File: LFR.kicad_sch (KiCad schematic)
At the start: 6 parts, among them M1 Motor_DC, M2 Motor_DC, U1 ESP32-S2-WROVER, U2 DRV8833PW

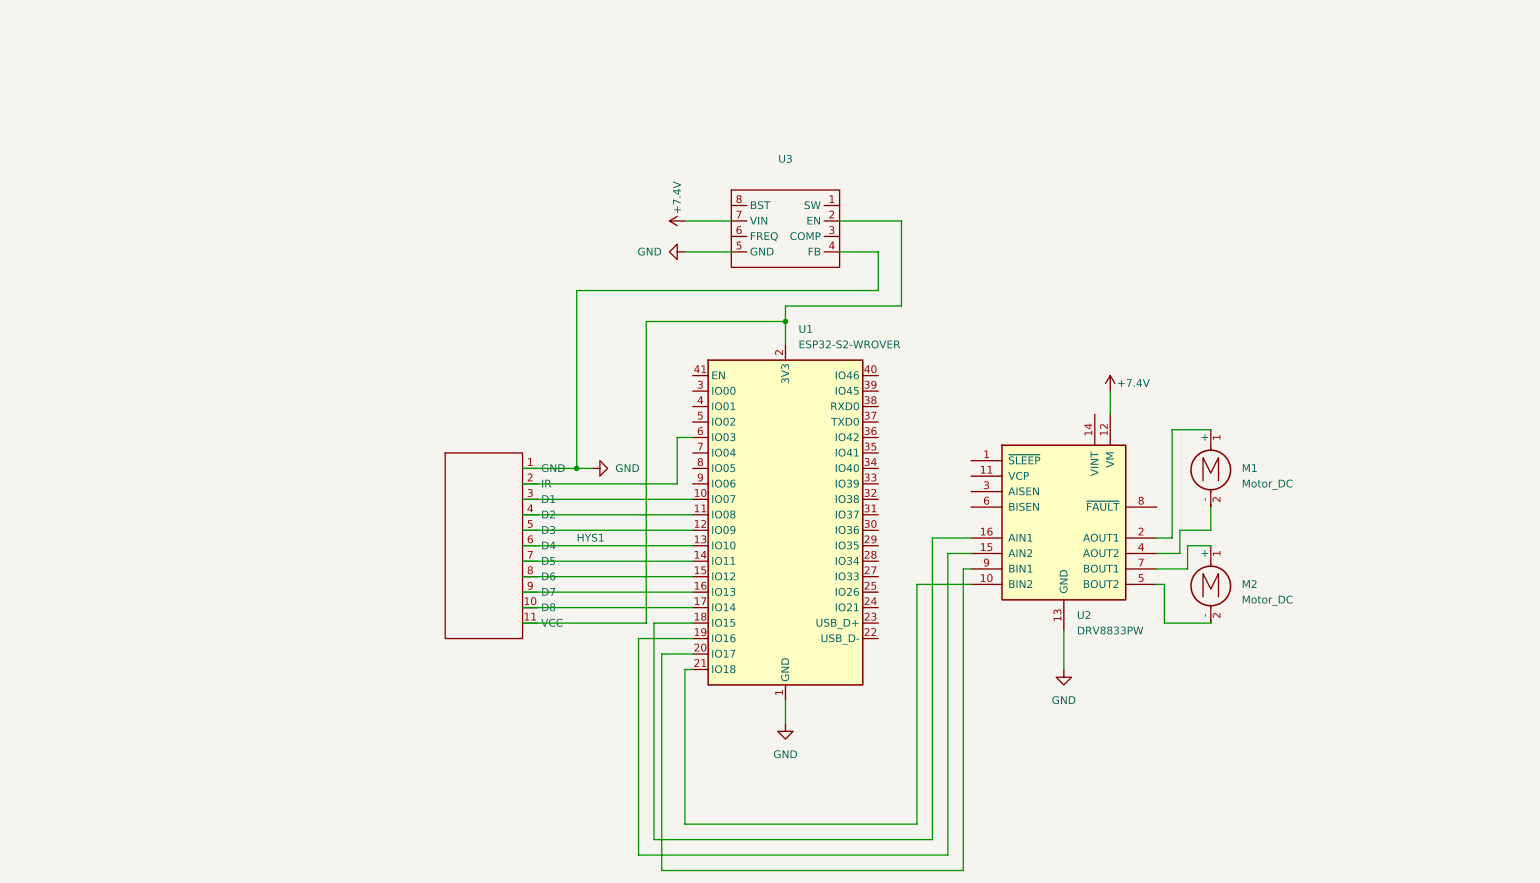
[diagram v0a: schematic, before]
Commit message: Add files via upload
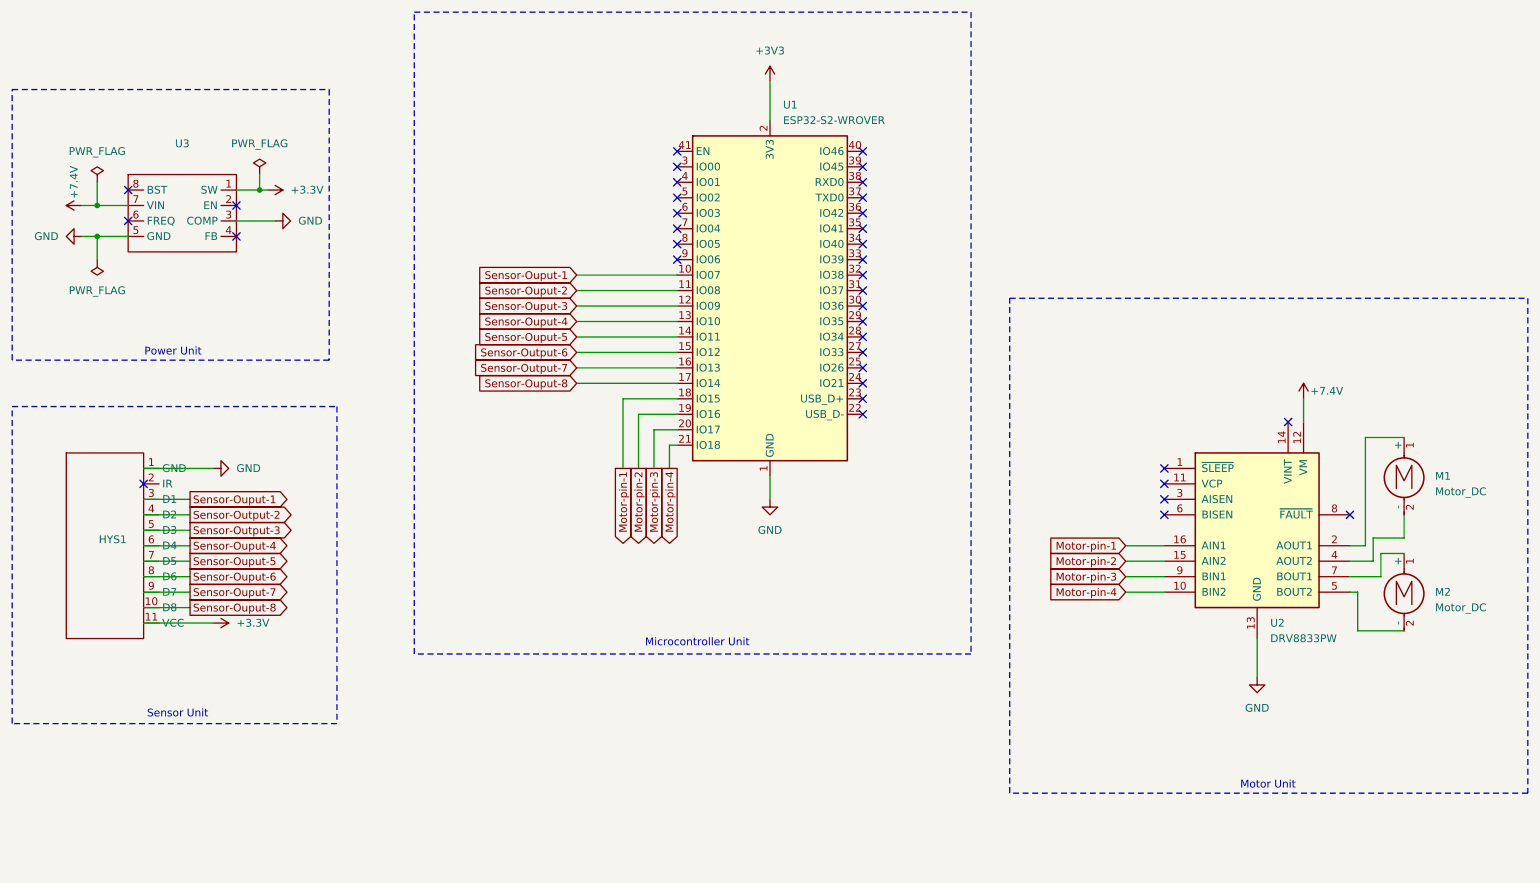
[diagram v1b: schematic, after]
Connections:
- net GND: now also U3.3 (COMP); no longer U3.4 (FB)
- net +3.3V: now reaches U3.1 (SW)
- net +3.3V: now also HYS1.11 (VCC)
- net Motor-pin-4: now reaches U1.21 (IO18), U2.10 (BIN2)
- net Motor-pin-2: now reaches U1.19 (IO16), U2.15 (AIN2)
- net Motor-pin-1: now reaches U1.18 (IO15), U2.16 (AIN1)
- net Motor-pin-3: now reaches U1.20 (IO17), U2.9 (BIN1)
- net Sensor-Ouput-8: now reaches HYS1.10 (D8), U1.17 (IO14)
- net at HYS1.2 (IR): no longer U1.6 (IO03)
- net Sensor-Ouput-1: now reaches HYS1.3 (D1), U1.10 (IO07)
- net Sensor-Ouput-2: now reaches U1.11 (IO08)
- net Sensor-Ouput-2: no longer HYS1.4 (D2)
- net Sensor-Ouput-3: now reaches U1.12 (IO09)
- net Sensor-Ouput-3: no longer HYS1.5 (D3)
- net Sensor-Ouput-4: now reaches HYS1.6 (D4), U1.13 (IO10)
- net Sensor-Ouput-5: now reaches HYS1.7 (D5), U1.14 (IO11)
- net Sensor-Ouput-6: now reaches HYS1.8 (D6)
- net Sensor-Ouput-6: no longer U1.15 (IO12)
- net Sensor-Ouput-7: now reaches HYS1.9 (D7)
- net Sensor-Ouput-7: no longer U1.16 (IO13)
- new net +3V3: U1.2 (3V3)
- new net Sensor-Output-2: HYS1.4 (D2)
- new net Sensor-Output-3: HYS1.5 (D3)
- new net Sensor-Output-6: U1.15 (IO12)
- new net Sensor-Output-7: U1.16 (IO13)
- now unconnected: U3.2 (EN)
- no-connect marks 0 -> 37
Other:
- note added: "Microcontroller Unit"
- note added: "Motor Unit"
- note added: "Power Unit"
- note added: "Sensor Unit"
- moved on the sheet: HYS1, M1, M2, U1, U2, U3
